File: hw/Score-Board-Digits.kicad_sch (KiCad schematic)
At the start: 65 parts, among them J11 Conn_02x09_Odd_Even, J12 Conn_02x09_Odd_Even, J13 Conn_02x09_Odd_Even

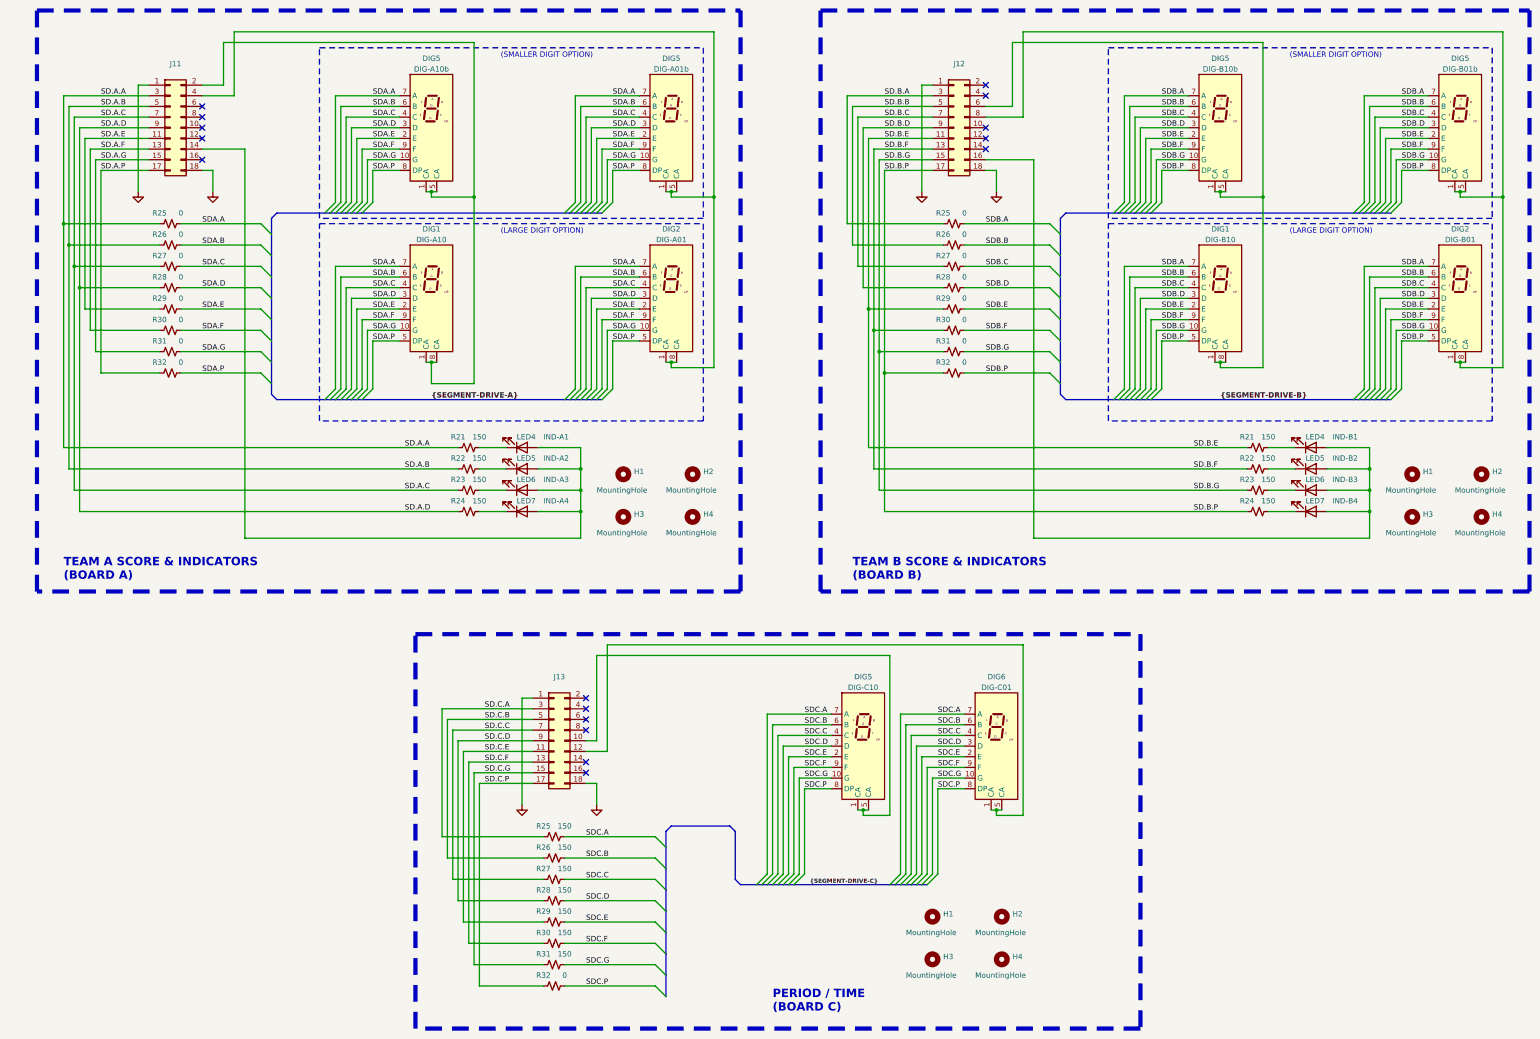
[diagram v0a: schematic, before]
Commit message: Digits schmatic ready for layout
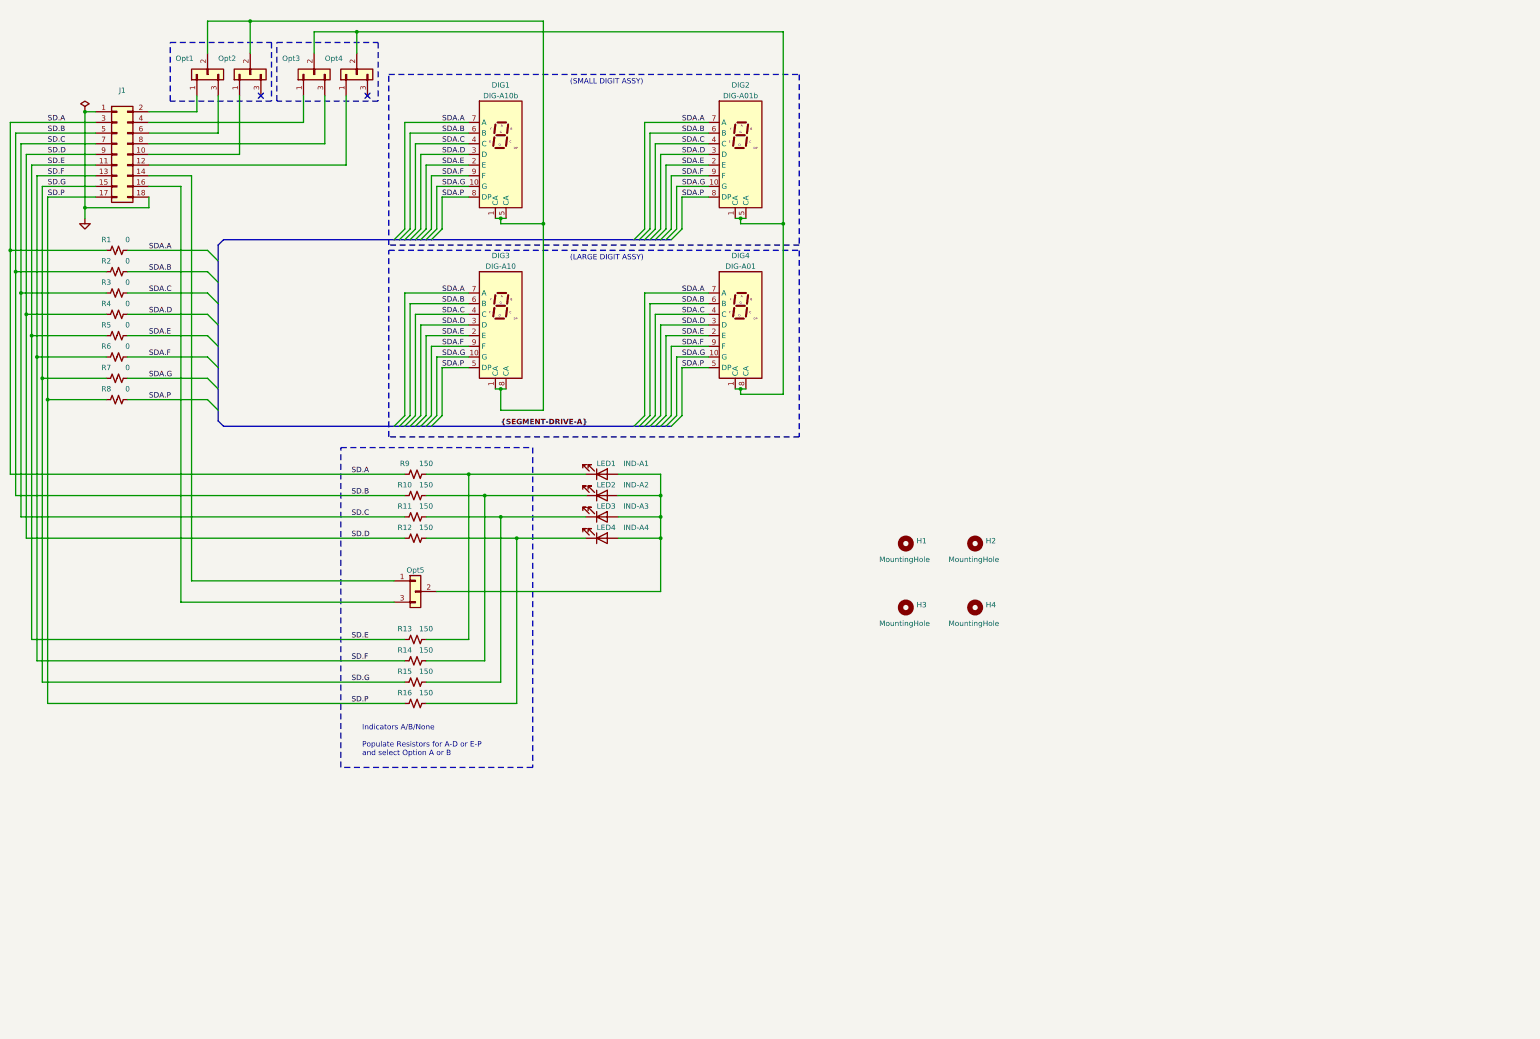
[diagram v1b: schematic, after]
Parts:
- removed DIG1, DIG2: WJLEDS40012TUR11, AES_Library:DISP-40101BCR-AES, symbol AES_Library:WJ-LEDS40012TUR11
- removed DIG5 (x3), DIG6: WJLEDS18012TUR11, AES_Library:DISP-CL18011BS-AES, symbol AES_Library:WJ-LEDS18012TUR11
- removed H1 (x2), H2 (x2), H3 (x2), H4 (x2): MountingHole, MountingHole:MountingHole_3.2mm_M3, symbol Mechanical:MountingHole
- removed J12, J13: Conn_02x09_Odd_Even, Connector_PinHeader_2.54mm:PinHeader_2x09_P2.54mm_Vertical, symbol Connector_Generic:Conn_02x09_Odd_Even
- removed LED4: IND-B1, LED_THT:LED_D5.0mm-3, symbol Device:LED
- removed LED5: IND-B2, LED_THT:LED_D5.0mm-3, symbol Device:LED
- removed LED6: IND-B3, LED_THT:LED_D5.0mm-3, symbol Device:LED
- removed LED7: IND-B4, LED_THT:LED_D5.0mm-3, symbol Device:LED
- removed R25, R26, R27, R28, R29, R30, R31: 150, Resistor_THT:R_Axial_DIN0207_L6.3mm_D2.5mm_P10.16mm_Horizontal, symbol Device:R_Small_US
- removed R25, R26, R27, R28, R29, R30, R31, R32 (x2): 0, Resistor_THT:R_Axial_DIN0207_L6.3mm_D2.5mm_P10.16mm_Horizontal, symbol Device:R_Small_US
- added Opt1, Opt2, Opt3, Opt4, Opt5: Opt_1-2, Connector_PinHeader_2.54mm:PinHeader_1x03_P2.54mm_Vertical, symbol AES_Library:Opt_1_of_2
- DIG1: renamed from DIG5; footprint AES_Library:DISP-CL18011BS-AES -> Connector_PinHeader_2.54mm:PinHeader_1x03_P2.54mm_Vertical
- renumbered DIG5 to DIG2, DIG1 to DIG3, DIG2 to DIG4, J11 to J1, LED4 to LED1, LED5 to LED2, LED6 to LED3, LED7 to LED4, R25 to R1, R22 to R10, R23 to R11, R24 to R12, R21 to R13, R22 to R14, R23 to R15, R24 to R16, R26 to R2, R27 to R3, R28 to R4, R29 to R5, R30 to R6, R31 to R7, R32 to R8, R21 to R9
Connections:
- net SD.B.E is gone; now on net SD.E: R13.1
- net SD.B.F is gone; now on net SD.F: R14.1
- net SD.B.G is gone; now on net SD.G: R15.1
- net SD.B.P is gone; now on net SD.P: R16.1
- net at DIG2.1 (CA), DIG2.5 (CA), DIG4.1 (CA)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: now also Opt3.2 (Pin_Common), Opt4.2 (Pin_Common); no longer J1.4 (Pin_4)
- net at R13.2: now also LED1.1 (K), R9.2
- net at R16.2: now also LED4.1 (K), R12.2
- net at LED3.1 (K), R11.2: now also R15.2
- net at DIG1.1 (CA), DIG1.5 (CA), DIG3.1 (CA)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: now also Opt1.2 (Pin_Common), Opt2.2 (Pin_Common); no longer J1.2 (Pin_2)
- net at R14.2: now also LED2.1 (K), R10.2
- net at LED1.2 (A), LED2.2 (A), LED3.2 (A)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: now also Opt5.2 (Pin_Common); no longer J1.14 (Pin_14)
- net at J1.10 (Pin_10): now also Opt2.1 (Pin_A)
- net at J1.12 (Pin_12): now also Opt4.1 (Pin_A)
- net at J1.16 (Pin_16): now also Opt5.3 (Pin_B)
- net at J1.6 (Pin_6): now also Opt1.3 (Pin_B)
- net at J1.8 (Pin_8): now also Opt3.3 (Pin_B)
- net SD.A.A renamed SD.A
- net SD.A.B renamed SD.B
- net SD.A.C renamed SD.C
- net SD.A.D renamed SD.D
- net SD.A.E renamed SD.E
- net SD.A.F renamed SD.F
- net SD.A.G renamed SD.G
- net SD.A.P renamed SD.P
- new net: J1.4 (Pin_4), Opt3.1 (Pin_A)
- new net: J1.2 (Pin_2), Opt1.1 (Pin_A)
- new net: J1.14 (Pin_14), Opt5.1 (Pin_A)
- no-connect marks 16 -> 2
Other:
- note added: "(LARGE DIGIT ASSY)"
- note added: "(SMALL DIGIT ASSY)"
- note added: "Indicators A/B/None Populate Resistors for A-D or E-P and select Option A or B"
- note removed: "(LARGE DIGIT OPTION)"
- note removed: "(SMALLER DIGIT OPTION)"
- note removed: "PERIOD / TIME (BOARD C)"
- note removed: "TEAM A SCORE & INDICATORS (BOARD A)"
- note removed: "TEAM B SCORE & INDICATORS (BOARD B)"
- moved on the sheet: DIG1, DIG2, DIG3, DIG4, H1, H2, H3, H4, J1, LED1, LED2, LED3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
